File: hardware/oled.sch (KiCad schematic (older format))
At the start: 2 parts, among them J1 SSD1306-OLED-SPI, U2 SSD1306-OLED-I2C

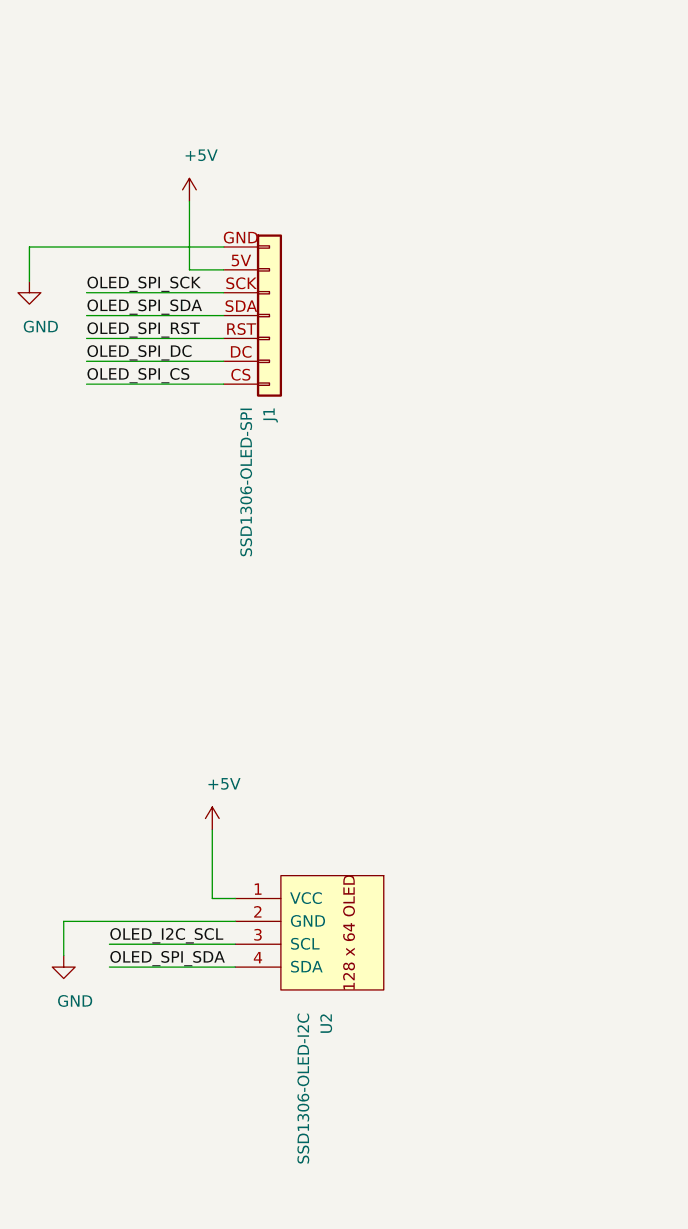
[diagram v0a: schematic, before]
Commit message: update,
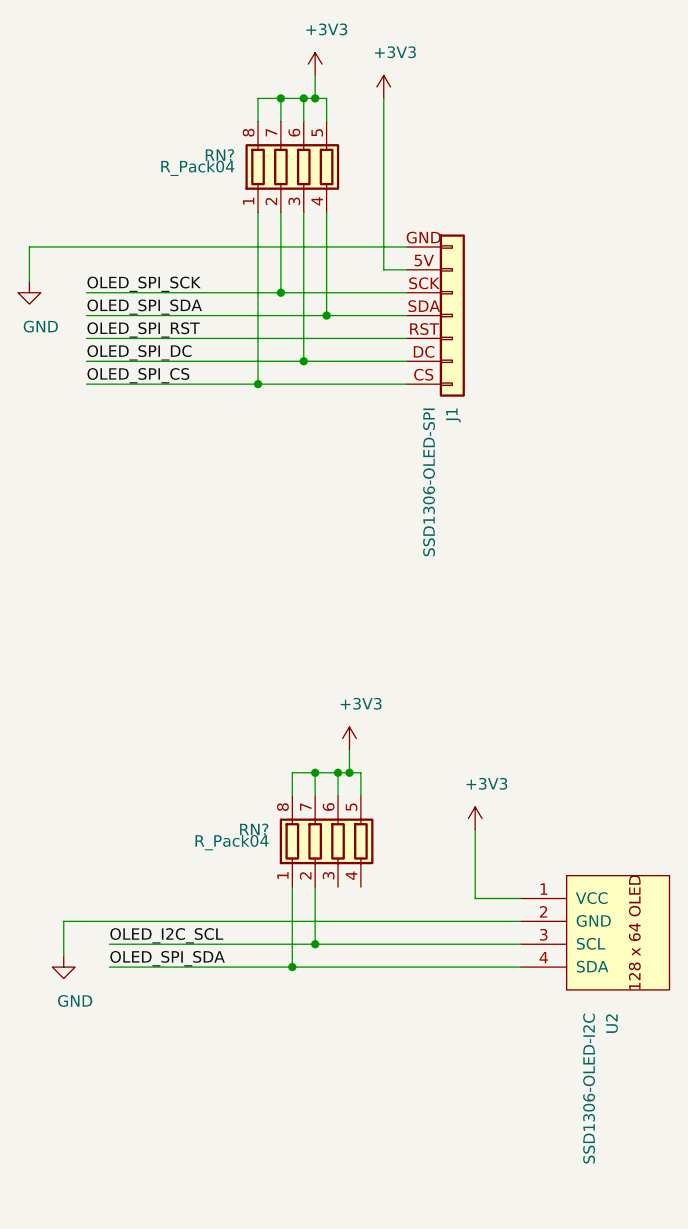
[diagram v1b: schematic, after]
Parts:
- added RN? (x2): R_Pack04, Resistor_SMD:R_Array_Concave_4x0603, symbol Device:R_Pack04
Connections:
- net OLED_I2C_SCL: now also RN?.2 (R2.1)
- net OLED_SPI_CS: now also RN?.1 (R1.1)
- net OLED_SPI_DC: now also RN?.3 (R3.1)
- net OLED_SPI_SCK: now also RN?.2 (R2.1)
- net OLED_SPI_SDA: now also RN?.1 (R1.1), RN?.4 (R4.1)
- net +5V renamed +3V3
- net +3V3: now also RN?.5 (R4.2), RN?.5 (R4.2), RN?.6 (R3.2), RN?.6 (R3.2), RN?.7 (R2.2), RN?.7 (R2.2), RN?.8 (R1.2), RN?.8 (R1.2)
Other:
- moved on the sheet: J1, U2
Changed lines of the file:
@@
 L taobao-components:SSD1306-OLED-SPI J1
 U 1 1 5CE3BBF1
-P 4850 2500
-F 0 "J1" V 4850 2100 50  0000 R CNN
-F 1 "SSD1306-OLED-SPI" V 4750 2100 50  0000 R CNN
-F 2 "footprint-lib:CONN_SPI_SSD1306" H 4850 2500 50  0001 C CNN
-F 3 "~" H 4850 2500 50  0001 C CNN
-	1    4850 2500
+P 5650 2500
+F 0 "J1" V 5650 2100 50  0000 R CNN
+F 1 "SSD1306-OLED-SPI" V 5550 2100 50  0000 R CNN
+F 2 "footprint-lib:CONN_SPI_SSD1306" H 5650 2500 50  0001 C CNN
+F 3 "~" H 5650 2500 50  0001 C CNN
+	1    5650 2500
 	1    0    0    -1
 $EndComp
@@
 L taobao-components:SSD1306-OLED-I2C U2
 U 1 1 5CE41586
-P 4800 5200
-F 0 "U2" H 5150 5500 50  0000 L CNN
-F 1 "SSD1306-OLED-I2C" H 5150 5400 50  0000 L CNN
-F 2 "footprint-lib:CONN_I2C_SSD1306" H 4800 4600 50  0001 C CNN
-F 3 "" H 4800 4600 50  0001 C CNN
-	1    4800 5200
+P 6050 5200
+F 0 "U2" H 6400 5500 50  0000 L CNN
+F 1 "SSD1306-OLED-I2C" H 6400 5400 50  0000 L CNN
+F 2 "footprint-lib:CONN_I2C_SSD1306" H 6050 4600 50  0001 C CNN
+F 3 "" H 6050 4600 50  0001 C CNN
+	1    6050 5200
 	0    1    1    0
 $EndComp
@@
 $EndComp
 Wire Wire Line
-	4650 2200 3800 2200
+	5450 2200 3800 2200
 Wire Wire Line
 	3800 2200 3800 2350
-$Comp
-L power:+5V #PWR?
-U 1 1 5CF7A062
-P 4500 2000
-F 0 "#PWR?" H 4500 1850 50  0001 C CNN
-F 1 "+5V" H 4550 2200 50  0000 C CNN
-F 2 "" H 4500 2000 50  0001 C CNN
-F 3 "" H 4500 2000 50  0001 C CNN
-	1    4500 2000
-	1    0    0    -1
-$EndComp
-Wire Wire Line
-	4500 2000 4500 2300
-Wire Wire Line
-	4500 2300 4650 2300
+Wire Wire Line
+	5350 1550 5350 2300
+Wire Wire Line
+	5350 2300 5450 2300
 Text Label 4050 2400 0    50   ~ 0
 OLED_SPI_SCK
@@
 OLED_SPI_CS
 Wire Wire Line
-	4050 2400 4650 2400
-Wire Wire Line
-	4050 2500 4650 2500
-Wire Wire Line
-	4050 2600 4650 2600
-Wire Wire Line
-	4050 2700 4650 2700
-Wire Wire Line
-	4050 2800 4650 2800
-$Comp
-L power:+5V #PWR?
-U 1 1 5CF7B0E0
-P 4600 4750
-F 0 "#PWR?" H 4600 4600 50  0001 C CNN
-F 1 "+5V" H 4650 4950 50  0000 C CNN
-F 2 "" H 4600 4750 50  0001 C CNN
-F 3 "" H 4600 4750 50  0001 C CNN
-	1    4600 4750
-	1    0    0    -1
-$EndComp
-Wire Wire Line
-	4600 4750 4600 5050
-Wire Wire Line
-	4700 5050 4600 5050
+	4050 2400 4900 2400
+Wire Wire Line
+	4050 2600 5450 2600
+Wire Wire Line
+	4050 2700 5000 2700
+Wire Wire Line
+	4050 2800 4800 2800
+Wire Wire Line
+	5750 4750 5750 5050
+Wire Wire Line
+	5950 5050 5750 5050
 $Comp
 L power:GND #PWR?
@@
 	3950 5300 3950 5150
 Wire Wire Line
-	3950 5150 4700 5150
+	3950 5150 5950 5150
 Text Label 4150 5250 0    50   ~ 0
 OLED_I2C_SCL
@@
 OLED_SPI_SDA
 Wire Wire Line
-	4150 5250 4700 5250
-Wire Wire Line
-	4150 5350 4700 5350
+	4150 5250 5050 5250
+Wire Wire Line
+	4150 5350 4950 5350
+$Comp
+L Device:R_Pack04 RN?
+U 1 1 5CF7E36C
+P 5000 1850
+AR Path="/5CDAB83A/5CF7E36C" Ref="RN?"  Part="1"
+AR Path="/5CDAB790/5CF7E36C" Ref="RN?"  Part="1"
+F 0 "RN?" H 4700 1900 50  0000 R CNN
+F 1 "R_Pack04" H 4700 1850 50  0000 R CNN
+F 2 "Resistor_SMD:R_Array_Concave_4x0603" V 5275 1850 50  0001 C CNN
+F 3 "~" H 5000 1850 50  0001 C CNN
+	1    5000 1850
+	1    0    0    -1
+$EndComp
+Wire Wire Line
+	5050 1450 5050 1550
+Wire Wire Line
+	5050 1550 5000 1550
+Wire Wire Line
+	4800 1550 4800 1650
+Wire Wire Line
+	4900 1650 4900 1550
+Connection ~ 4900 1550
+Wire Wire Line
+	4900 1550 4800 1550
+Wire Wire Line
+	5000 1550 5000 1650
+Connection ~ 5000 1550
+Wire Wire Line
+	5000 1550 4900 1550
+Wire Wire Line
+	5100 1650 5100 1550
+Wire Wire Line
+	5100 1550 5050 1550
+Connection ~ 5050 1550
+Wire Wire Line
+	4800 2050 4800 2800
+Connection ~ 4800 2800
+Wire Wire Line
+	4800 2800 5450 2800
+Wire Wire Line
+	4900 2050 4900 2400
+Connection ~ 4900 2400
+Wire Wire Line
+	4900 2400 5450 2400
+Wire Wire Line
+	4050 2500 5100 2500
+Wire Wire Line
+	5000 2050 5000 2700
+Connection ~ 5000 2700
+Wire Wire Line
+	5000 2700 5450 2700
+Wire Wire Line
+	5100 2050 5100 2500
+Connection ~ 5100 2500
+Wire Wire Line
+	5100 2500 5450 2500
+$Comp
+L Device:R_Pack04 RN?
+U 1 1 5CF83F57
+P 5150 4800
+AR Path="/5CDAB83A/5CF83F57" Ref="RN?"  Part="1"
+AR Path="/5CDAB790/5CF83F57" Ref="RN?"  Part="1"
+F 0 "RN?" H 4850 4850 50  0000 R CNN
+F 1 "R_Pack04" H 4850 4800 50  0000 R CNN
+F 2 "Resistor_SMD:R_Array_Concave_4x0603" V 5425 4800 50  0001 C CNN
+F 3 "~" H 5150 4800 50  0001 C CNN
+	1    5150 4800
+	1    0    0    -1
+$EndComp
+Wire Wire Line
+	5200 4400 5200 4500
+Wire Wire Line
+	5200 4500 5150 4500
+Wire Wire Line
+	4950 4500 4950 4600
+Wire Wire Line
+	5050 4600 5050 4500
+Connection ~ 5050 4500
+Wire Wire Line
+	5050 4500 4950 4500
+Wire Wire Line
+	5150 4500 5150 4600
+Connection ~ 5150 4500
+Wire Wire Line
+	5150 4500 5050 4500
+Wire Wire Line
+	5250 4600 5250 4500
+Wire Wire Line
+	5250 4500 5200 4500
+Connection ~ 5200 4500
+Wire Wire Line
+	4950 5000 4950 5350
+Connection ~ 4950 5350
+Wire Wire Line
+	4950 5350 5950 5350
+Wire Wire Line
+	5050 5000 5050 5250
+Connection ~ 5050 5250
+Wire Wire Line
+	5050 5250 5950 5250
+$Comp
+L power:+3V3 #PWR?
+U 1 1 5CF89EF6
+P 5050 1450
+F 0 "#PWR?" H 5050 1300 50  0001 C CNN
+F 1 "+3V3" H 5100 1650 50  0000 C CNN
+F 2 "" H 5050 1450 50  0001 C CNN
+F 3 "" H 5050 1450 50  0001 C CNN
+	1    5050 1450
+	1    0    0    -1
+$EndComp
+$Comp
+L power:+3V3 #PWR?
+U 1 1 5CF8A20A
+P 5350 1550
+F 0 "#PWR?" H 5350 1400 50  0001 C CNN
+F 1 "+3V3" H 5400 1750 50  0000 C CNN
+F 2 "" H 5350 1550 50  0001 C CNN
+F 3 "" H 5350 1550 50  0001 C CNN
+	1    5350 1550
+	1    0    0    -1
+$EndComp
+$Comp
+L power:+3V3 #PWR?
+U 1 1 5CF8A4BE
+P 5200 4400
+F 0 "#PWR?" H 5200 4250 50  0001 C CNN
+F 1 "+3V3" H 5250 4600 50  0000 C CNN
+F 2 "" H 5200 4400 50  0001 C CNN
+F 3 "" H 5200 4400 50  0001 C CNN
+	1    5200 4400
+	1    0    0    -1
+$EndComp
+$Comp
+L power:+3V3 #PWR?
+U 1 1 5CF8B0B2
+P 5750 4750
+F 0 "#PWR?" H 5750 4600 50  0001 C CNN
+F 1 "+3V3" H 5800 4950 50  0000 C CNN
+F 2 "" H 5750 4750 50  0001 C CNN
+F 3 "" H 5750 4750 50  0001 C CNN
+	1    5750 4750
+	1    0    0    -1
+$EndComp
 $EndSCHEMATC
